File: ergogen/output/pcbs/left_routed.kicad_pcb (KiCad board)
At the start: 2 copper layers, 140.9 x 96.1 mm, 88 parts

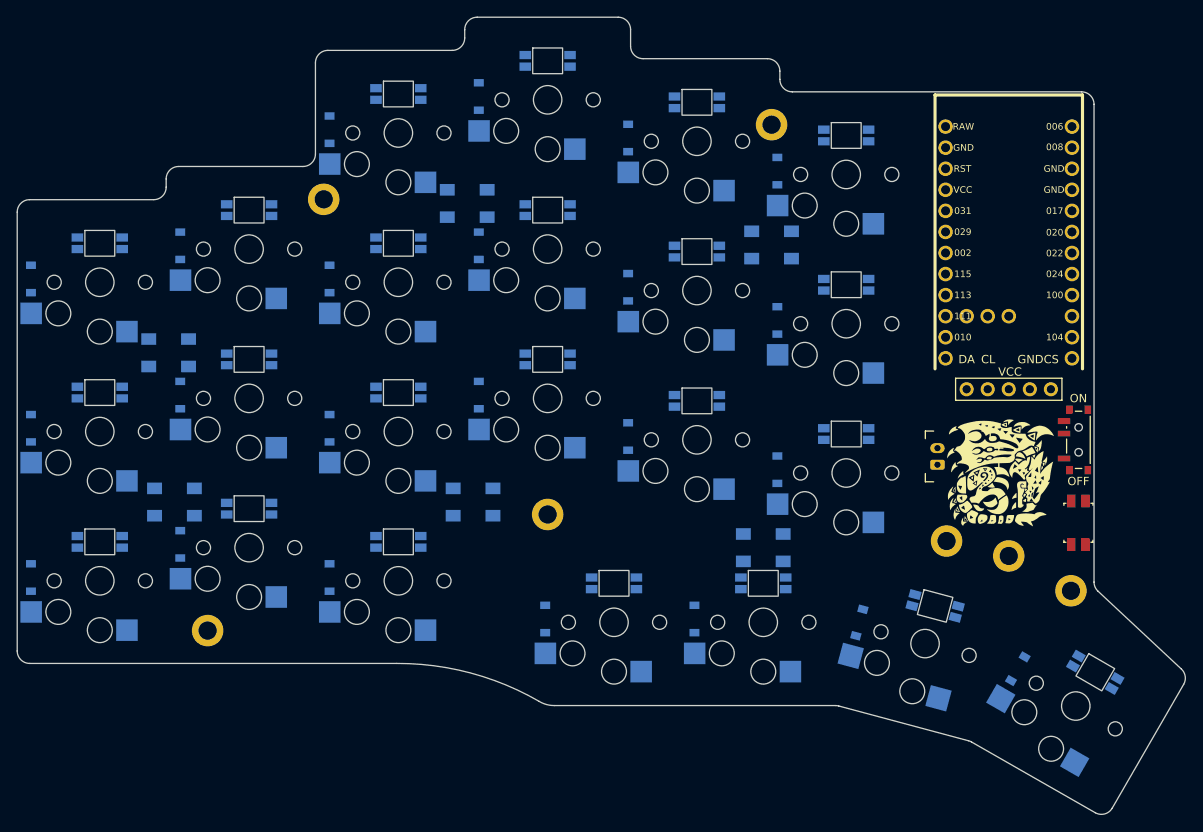
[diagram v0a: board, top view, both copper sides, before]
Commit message: add: generated files
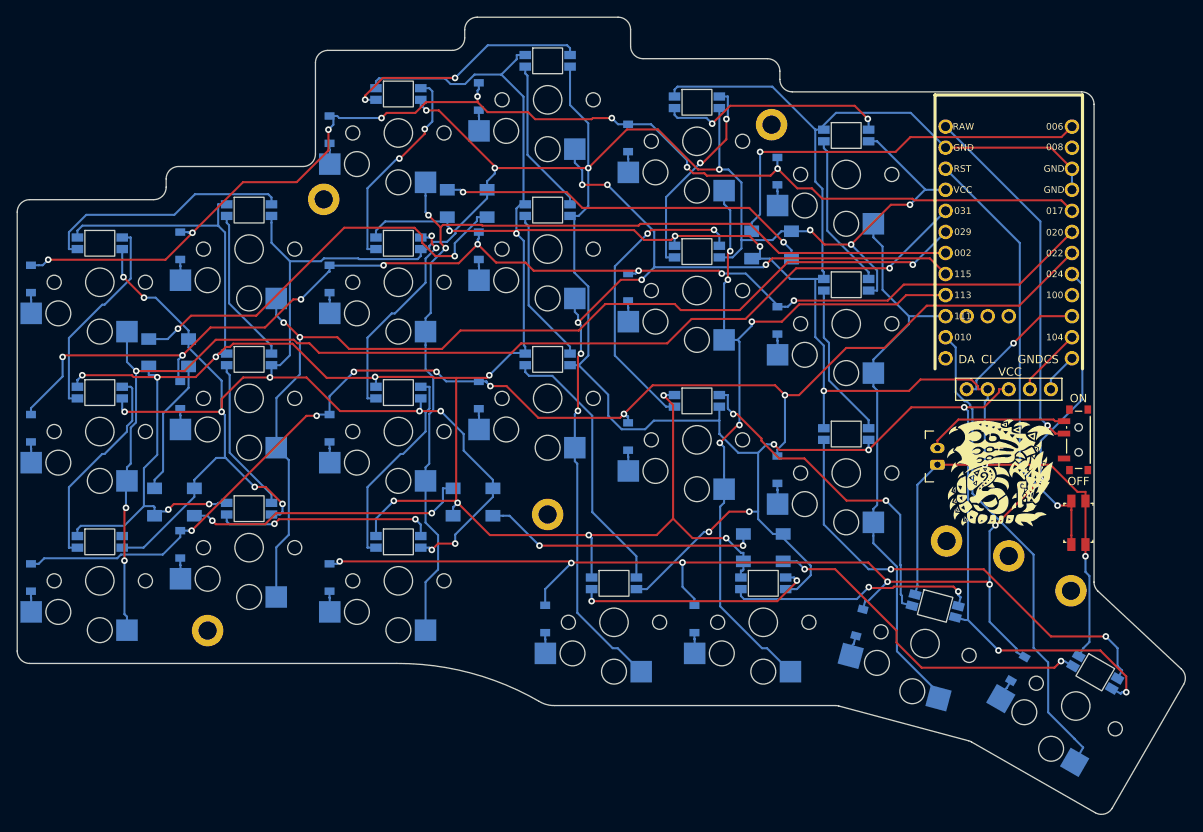
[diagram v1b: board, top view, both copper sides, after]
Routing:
- net GND: track 0.00 -> 534.9 mm, vias 0 -> 19
- net VCC: track 0.00 -> 497.9 mm, vias 0 -> 25
- net P022: track 0.00 -> 157.7 mm, vias 0 -> 7
- net P024: track 0.00 -> 151.0 mm, vias 0 -> 7
- net P020: track 0.00 -> 149.7 mm, vias 0 -> 8
- net P017: track 0.00 -> 148.4 mm, vias 0 -> 8
- net P031: track 0.00 -> 144.5 mm, vias 0 -> 4
- net P029: track 0.00 -> 124.9 mm, vias 0 -> 3
- net P002: track 0.00 -> 120.6 mm, vias 0 -> 2
- net P115: track 0.00 -> 117.6 mm, vias 0 -> 7
- net P113: track 0.00 -> 93.3 mm, vias 0 -> 5
- net P111: track 0.00 -> 68.8 mm
- net P010: track 0.00 -> 58.6 mm
- net LED_1: track 0.00 -> 55.8 mm, vias 0 -> 2
- net RST: track 0.00 -> 53.1 mm, vias 0 -> 1
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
